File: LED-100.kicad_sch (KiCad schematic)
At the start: 27 parts, among them J2 LDA100_2_J2, J3 LDA100_2_J3, J4 LDA100_2_J4, J5 xtra, J7 Conn_01x01, J8 Conn_01x07, SW2 SW_SPST, U1 TLC5947DAP, U2 TLC5947DAP, U3 TLC5947DAP, U4 TEENSY 4.0

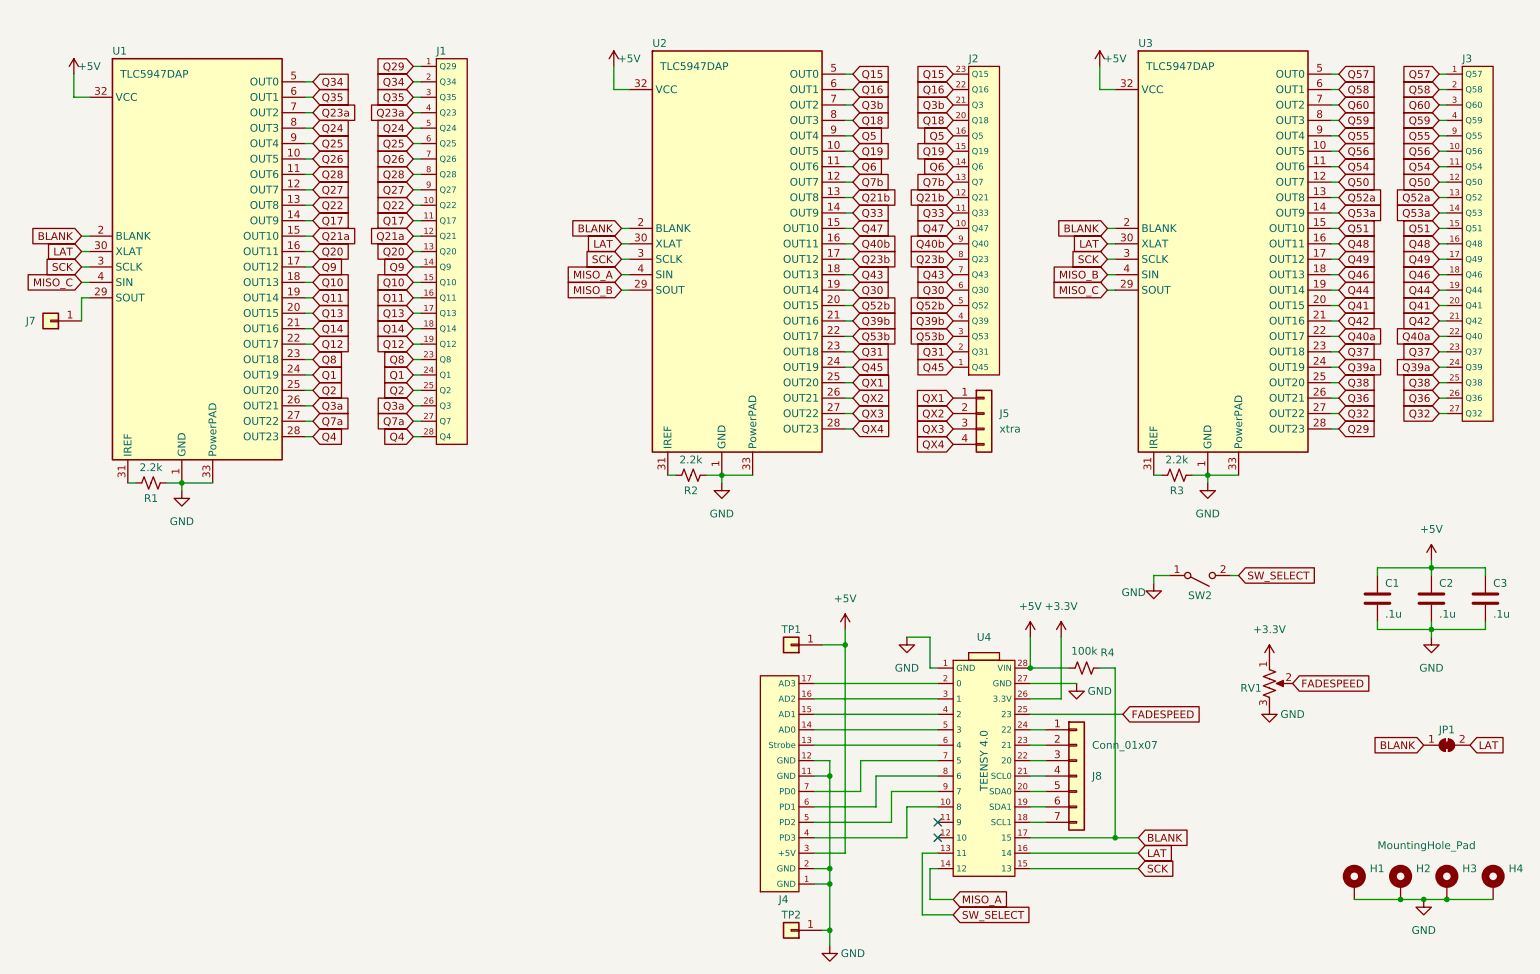
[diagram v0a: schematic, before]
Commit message: Rev 5
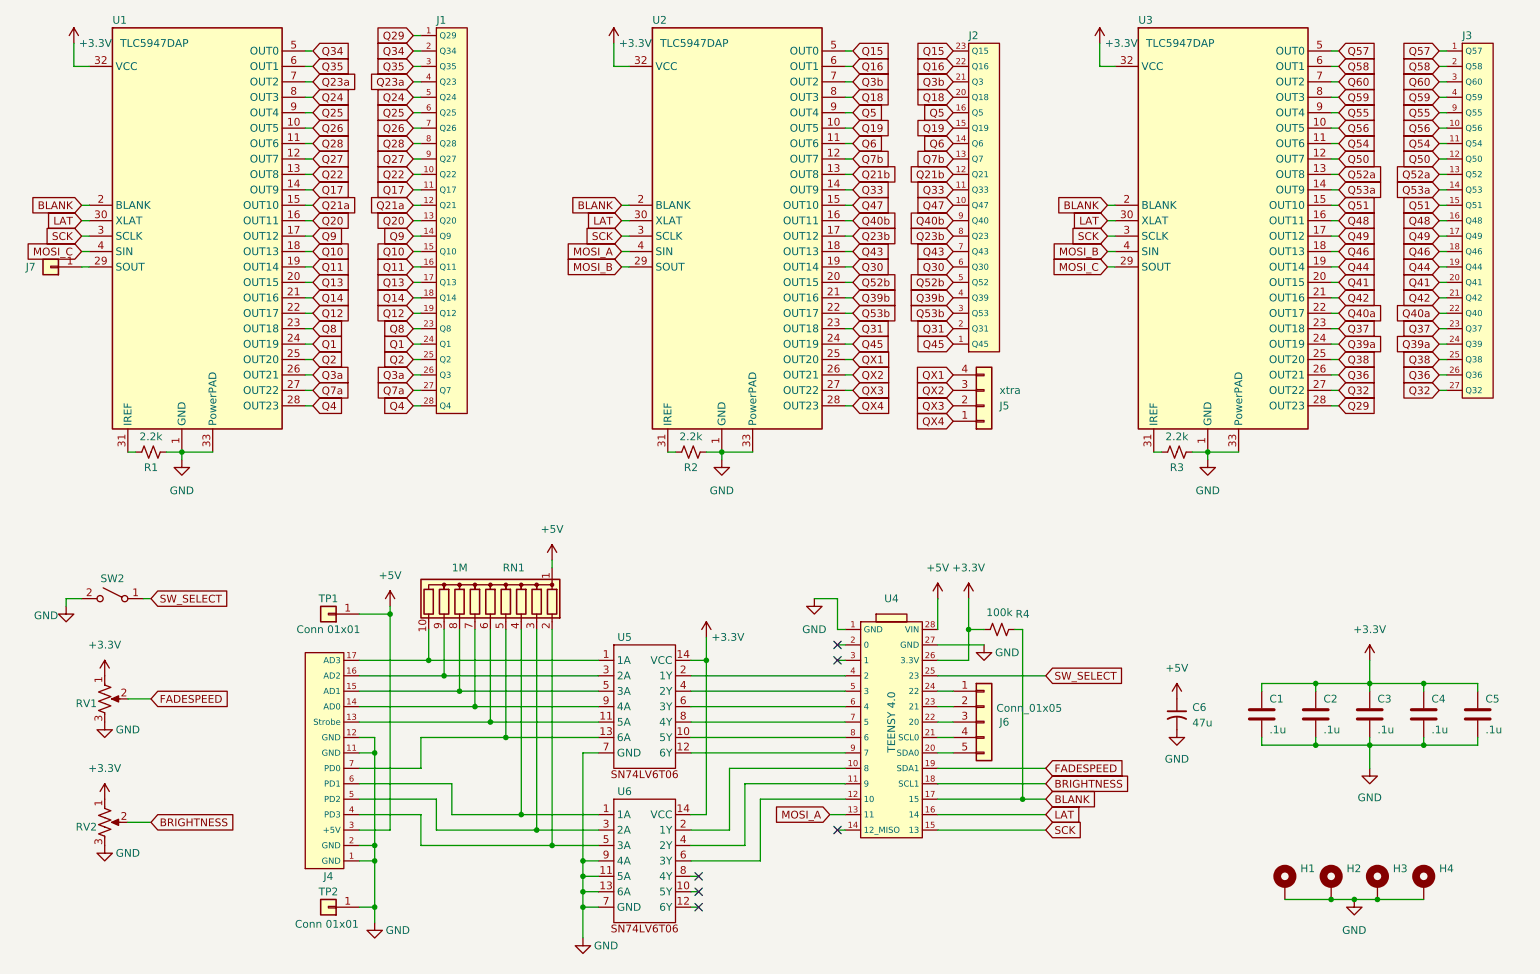
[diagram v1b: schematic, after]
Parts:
- removed JP1: SolderJumper_2_Bridged, Jumper:SolderJumper-2_P1.3mm_Bridged_Pad1.0x1.5mm, symbol Jumper:SolderJumper_2_Bridged
- added C4, C5: .1u, Capacitor_THT:C_Disc_D3.0mm_W1.6mm_P2.50mm, symbol Device:C
- added C6: 47u, Capacitor_THT:CP_Radial_D6.3mm_P2.50mm, symbol Device:C_Small_US
- added RN1: 1M, Resistor_THT:R_Array_SIP10, symbol Device:R_Network09
- added RV2: 100k, Potentiometer_THT:Potentiometer_Bourns_PTV09A-1_Single_Vertical, symbol Device:R_Potentiometer_US
- added U5, U6: (no value), Package_SO:TSSOP-14_4.4x5mm_P0.65mm, symbol Logic_LevelTranslator:SN74LV6T06
- C1, C2, C3: footprint Capacitor_THT:C_Disc_D3.0mm_W2.0mm_P2.50mm -> Capacitor_THT:C_Disc_D3.0mm_W1.6mm_P2.50mm
- J1: value ~ -> (none)
- J6: renamed from J8; value Conn_01x07 -> Conn_01x05; footprint Connector_PinHeader_2.54mm:PinHeader_1x07_P2.54mm_Vertical -> Connector_PinHeader_2.54mm:PinHeader_1x05_P2.54mm_Vertical; symbol Connector_Generic:Conn_01x07 -> Connector_Generic:Conn_01x05
- RV1: footprint Potentiometer_THT:Potentiometer_Piher_PT-10-V10_Vertical -> Potentiometer_THT:Potentiometer_Bourns_PTV09A-1_Single_Vertical
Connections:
- net +3.3V: now also C1.1, C2.1, C3.1, R4.1, U1.32 (VCC), U2.32 (VCC), U3.32 (VCC), C4.1, C5.1, RV2.1, U5.14 (VCC), U6.14 (VCC)
- net +5V: now also C6.1, RN1.1 (common); no longer C1.1, C2.1, C3.1, R4.1, U1.32 (VCC), U2.32 (VCC), U3.32 (VCC)
- net FADESPEED: now also U4.19 (SDA1); no longer U4.25 (23)
- net GND: now also SW2.2 (B), C4.2, C5.2, C6.2, RV2.3, U5.7 (GND), U6.11 (5A), U6.13 (6A), U6.7 (GND), U6.9 (4A); no longer SW2.1 (A)
- net QX1: now also J5.4 (Pin_4); no longer J5.1 (Pin_1)
- net QX2: now also J5.3 (Pin_3); no longer J5.2 (Pin_2)
- net QX3: now also J5.2 (Pin_2); no longer J5.3 (Pin_3)
- net QX4: now also J5.1 (Pin_1); no longer J5.4 (Pin_4)
- net SW_SELECT: now also SW2.1 (A), U4.25 (23); no longer SW2.2 (B), U4.13 (11)
- net at U4.10 (8): now also U6.2 (1Y); no longer J4.4 (PD3)
- net at U4.11 (9): now also U6.4 (2Y)
- net at U4.12 (10): now also U6.6 (3Y)
- net BRIGHTNESS: now reaches U4.18 (SCL1)
- net BRIGHTNESS: now also RV2.2; no longer J6.7 (Pin_7)
- net at U4.2 (0): no longer J4.17 (AD3)
- net at U4.3 (1): no longer J4.16 (AD2)
- net at U4.4 (2): now also U5.2 (1Y); no longer J4.15 (AD1)
- net at U4.5 (3): now also U5.4 (2Y); no longer J4.14 (AD0)
- net at U4.6 (4): now also U5.6 (3Y); no longer J4.13 (Strobe)
- net at U4.7 (5): now also U5.8 (4Y); no longer J4.7 (PD0)
- net at U4.8 (6): now also U5.10 (5Y); no longer J4.6 (PD1)
- net at U4.9 (7): now also U5.12 (6Y); no longer J4.5 (PD2)
- net MISO_A: no longer names the net of U4.14 (12_MISO)
- net MISO_A: no longer U2.4 (SIN)
- net MISO_B renamed MOSI_B
- net MISO_C renamed MOSI_C
- new net: J4.13 (Strobe), RN1.6 (R5), U5.11 (5A)
- new net: J4.14 (AD0), RN1.7 (R6), U5.9 (4A)
- new net: J4.15 (AD1), RN1.8 (R7), U5.5 (3A)
- new net: J4.16 (AD2), RN1.9 (R8), U5.3 (2A)
- new net: J4.17 (AD3), RN1.10 (R9), U5.1 (1A)
- new net: J4.4 (PD3), RN1.2 (R1), U6.5 (3A)
- new net: J4.5 (PD2), RN1.3 (R2), U6.3 (2A)
- new net: J4.6 (PD1), RN1.4 (R3), U6.1 (1A)
- new net: J4.7 (PD0), RN1.5 (R4), U5.13 (6A)
- new net MOSI_A: U2.4 (SIN), U4.13 (11)
- no-connect marks 2 -> 6
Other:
- moved on the sheet: C1, C2, C3, H1, H2, H3, H4, J1, J2, J3, J4, J5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
